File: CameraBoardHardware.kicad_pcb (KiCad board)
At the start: 2 copper layers, 44 parts, among them J1 BNC_75_OHM_HORIZ, U1 Picoblade_3, U10 LMH6574MA, U11 TM4C129E_Launchpad_X7, U12 TXB0102_DCU_8, U13 Molex_SL_3, U14 Picoblade_3, U2 Picoblade_3, U3 Picoblade_3, U4 Picoblade_3, U5 Molex_SL_3, U6 Molex_SL_3, U7 Molex_SL_3, U8 Molex_SL_3, U9 OKI

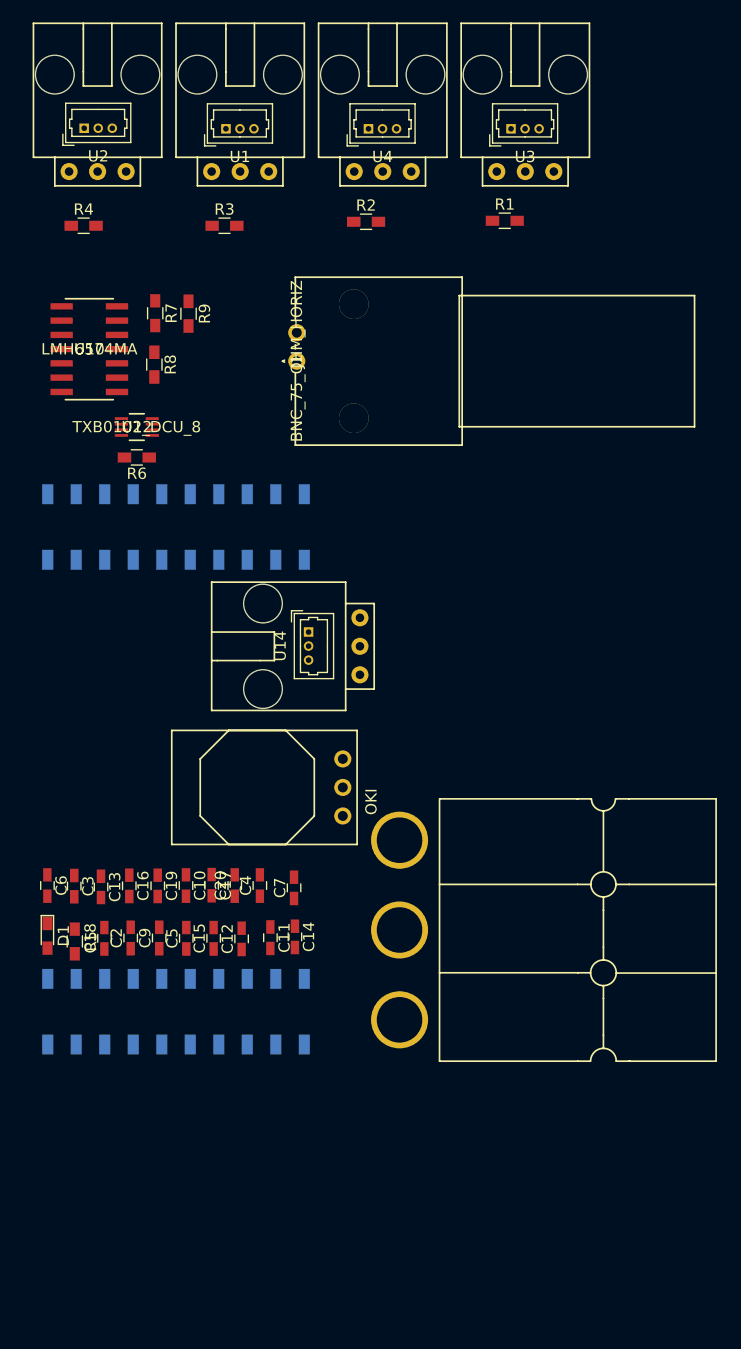
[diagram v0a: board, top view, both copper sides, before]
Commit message: Gerbs
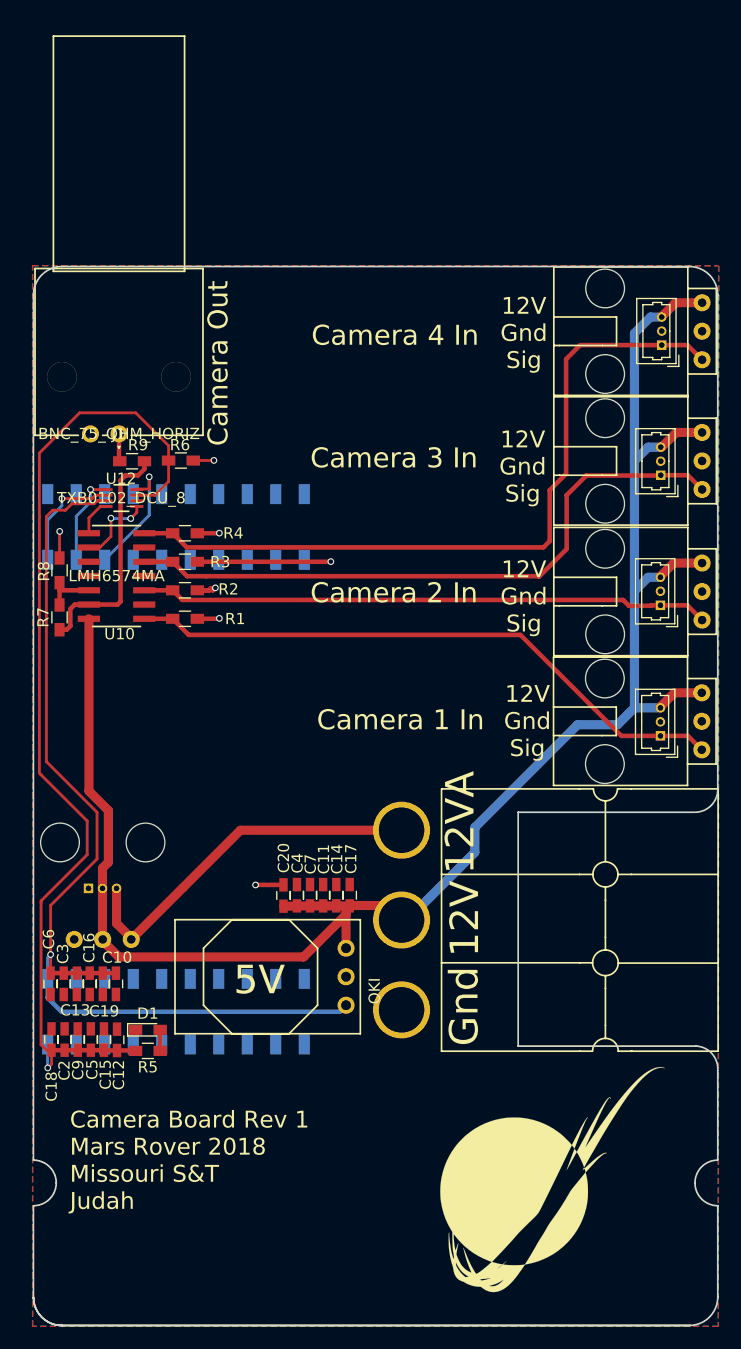
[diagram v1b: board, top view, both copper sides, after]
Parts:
- added G***: LOGO, MRDT_Silkscreens:Atlas_Logo_28.6mmX37.3mm, B.Cu at (140.9, 138.6)
- added G***: LOGO, MRDT_Silkscreens:MRDT_Logo_20mm, F.Cu at (156.1, 195.2)
- U13, U14: moved to B.Cu
- moved U4 60.0 mm to (165.7, 155.7), turned to 90 degrees
- moved U2 59.9 mm to (165.7, 132.5), turned to 90 degrees
- moved U5 55.7 mm to (169.4, 119.6), turned to 90 degrees
- moved U8 51.4 mm to (169.4, 154.4), turned to 90 degrees
- moved U6 48.6 mm to (169.4, 131.2), turned to 90 degrees
- moved U7 47.0 mm to (169.4, 142.8), turned to 90 degrees
- moved R1 45.5 mm to (123.4, 145.2)
- moved U3 44.5 mm to (165.7, 144.0), turned to 90 degrees
- moved U1 43.3 mm to (165.8, 120.9), turned to 90 degrees
- moved R2 36.6 mm to (123.4, 142.7)
- moved U13 34.7 mm to (116.0, 173.8), turned to 180 degrees
- moved R3 30.1 mm to (123.4, 140.2)
- moved U14 30.1 mm to (114.8, 169.3), turned to 0 degrees
- moved R4 28.8 mm to (123.4, 137.6)
- moved R7 28.4 mm to (112.2, 145.1), turned to 90 degrees
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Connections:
- R6 pad 2: OE -> 3.3V
- U10 pad 8: A0 -> B1
- U10 pad 9: A1 -> B2
- U12 pad 1: B1 -> B2
- U12 pad 2: 5V -> Gnd
- U12 pad 3: OE -> 3.3V
- U12 pad 4: A1 -> A2
- U12 pad 5: A2 -> A1
- U12 pad 6: 3.3V -> OE
- U12 pad 7: Gnd -> 5V
- U12 pad 8: B2 -> B1
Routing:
- net 12V: track 0.00 -> 159.8 mm
- net 3.3V: track 0.00 -> 89.6 mm, vias 0 -> 1
- net 5V: track 0.00 -> 87.9 mm, vias 0 -> 1
- net Camera4_In: track 0.00 -> 66.8 mm
- net Camera3_In: track 0.00 -> 57.3 mm
- net Camera1_In: track 0.00 -> 54.5 mm
- net Camera2_In: track 0.00 -> 50.8 mm
- net 12VA: track 0.00 -> 33.2 mm
- net Gnd: track 0.00 -> 25.5 mm, vias 0 -> 7
- net Net-(R7-Pad1): track 0.00 -> 21.4 mm
- net A2: track 0.00 -> 11.2 mm, vias 0 -> 1
- net OE: track 0.00 -> 10.0 mm, vias 0 -> 1
- net A1: track 0.00 -> 8.17 mm, vias 0 -> 1
- net B2: track 0.00 -> 7.07 mm, vias 0 -> 2
- net Net-(R7-Pad2): track 0.00 -> 4.61 mm
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- added copper zone on B.Cu, net Gnd
- added copper zone on F.Cu, net Gnd
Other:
- board outline added: 61 x 94.3 mm
- board text added: "12V"
- board text added: "12V Act"
- board text added: "12V Gnd Sig"
- board text added: "12VA"
- board text added: "12VA 12V Gnd"
- board text added: "5V"
- board text added: "Camera 1 In"
- board text added: "Camera 2 In"
- board text added: "Camera 3 In"
- board text added: "Camera 4 In"
- board text added: "Camera Board Rev 1 Mars Rover 2018 Missouri S&T Judah"
- board text added: "Camera Out"
- board text added: "Gnd"
